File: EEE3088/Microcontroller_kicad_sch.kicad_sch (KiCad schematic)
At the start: 1 part, among them U1 STM32F051C6Tx

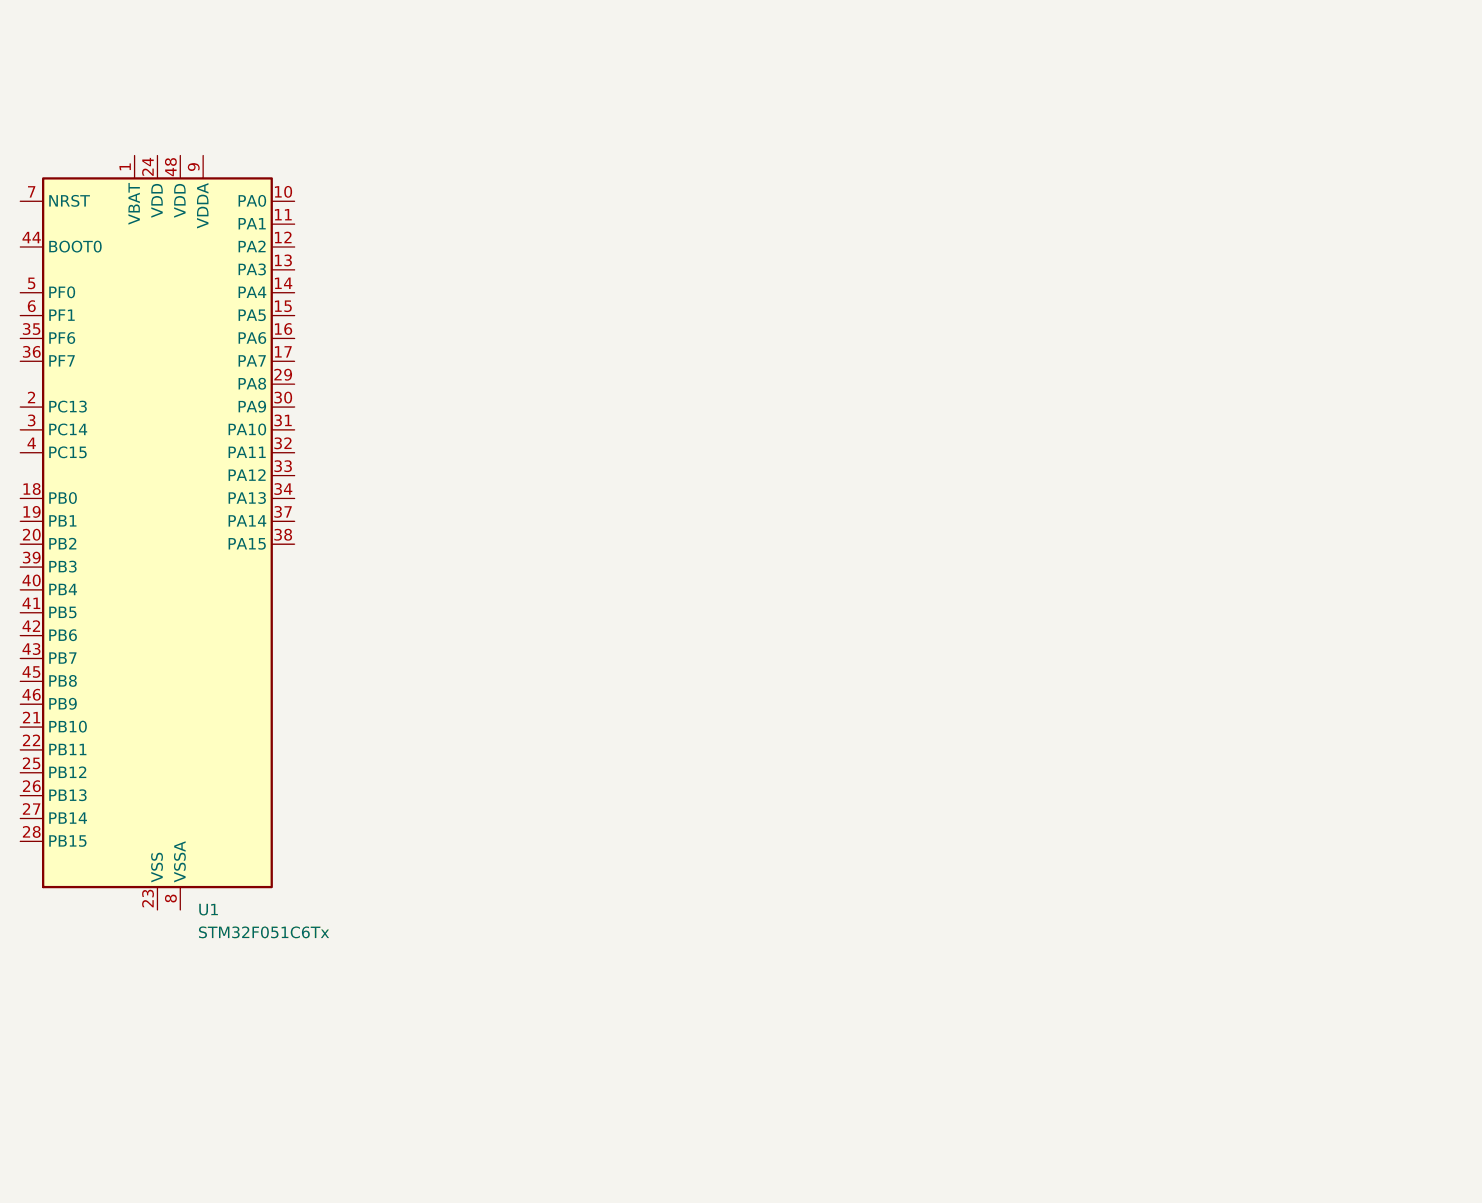
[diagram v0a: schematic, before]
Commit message: First night - c
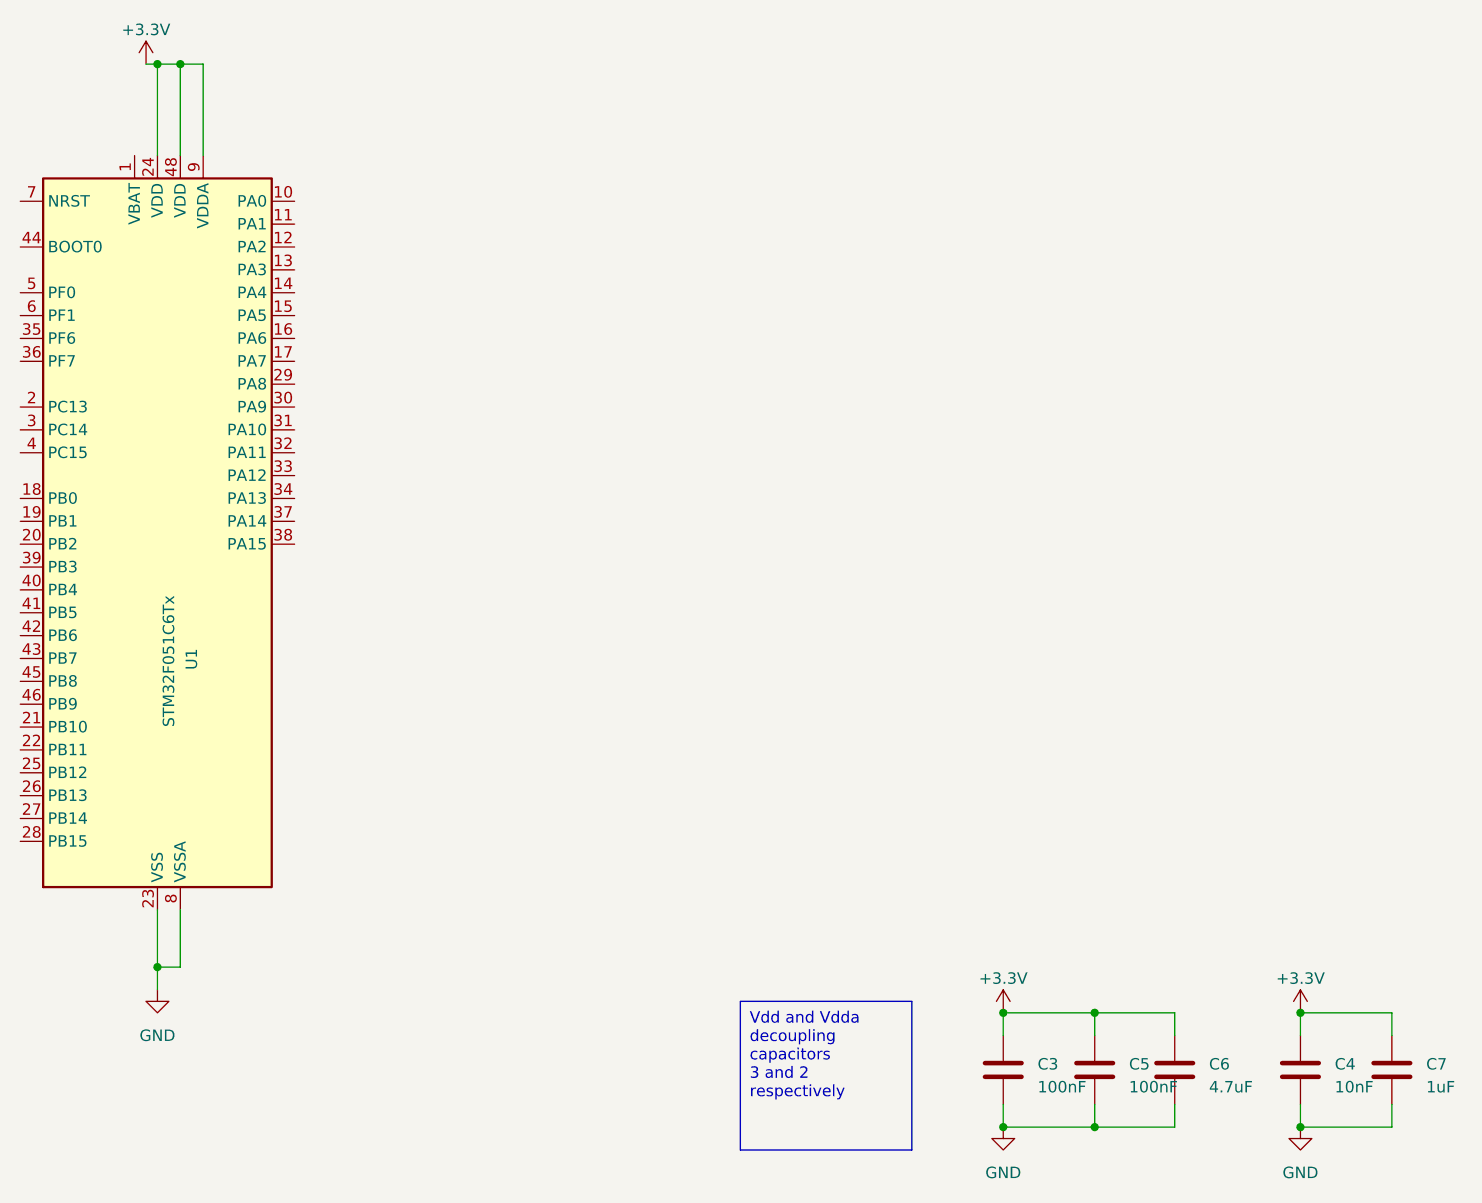
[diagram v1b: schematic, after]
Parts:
- added C3, C5: 100nF, symbol Device:C
- added C4: 10nF, symbol Device:C
- added C6: 4.7uF, symbol Device:C
- added C7: 1uF, symbol Device:C
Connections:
- net GND: now reaches U1.23 (VSS), U1.47 (VSS)
- net GND: now also U1.8 (VSSA), C3.2, C4.2, C5.2, C6.2, C7.2
- net +3.3V: now reaches U1.24 (VDD)
- net +3.3V: now also U1.48 (VDD), U1.9 (VDDA), C3.1, C4.1, C5.1, C6.1, C7.1
